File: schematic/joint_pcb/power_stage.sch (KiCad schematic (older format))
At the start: 36 parts, among them J2 Amp_Power, J3 Audio OUTPUT, Q1 IRF530A, Q2 IRF530A, Q3 IRF530A, Q4 IRF530A, U3 HIP4082IP

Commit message: Fixed PCB
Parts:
- Q1, Q2, Q3, Q4: symbol dk_Transistors-FETs-MOSFETs-Single:IRF540NPBF -> joint_pcb-rescue:IRF540NPBF-dk_Transistors-FETs-MOSFETs-Single
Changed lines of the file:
@@
 	3000 4350 3100 4350
 $Comp
-L dk_Transistors-FETs-MOSFETs-Single:IRF540NPBF Q2
+L joint_pcb-rescue:IRF540NPBF-dk_Transistors-FETs-MOSFETs-Single Q2
 U 1 1 61356BCC
 P 6500 4350
@@
 	4350 3950 5700 3950
 $Comp
-L dk_Transistors-FETs-MOSFETs-Single:IRF540NPBF Q3
+L joint_pcb-rescue:IRF540NPBF-dk_Transistors-FETs-MOSFETs-Single Q3
 U 1 1 61314458
 P 9650 2950
@@
 $EndComp
 $Comp
-L dk_Transistors-FETs-MOSFETs-Single:IRF540NPBF Q4
+L joint_pcb-rescue:IRF540NPBF-dk_Transistors-FETs-MOSFETs-Single Q4
 U 1 1 6132015F
 P 9650 4350
@@
 $EndComp
 $Comp
-L dk_Transistors-FETs-MOSFETs-Single:IRF540NPBF Q1
+L joint_pcb-rescue:IRF540NPBF-dk_Transistors-FETs-MOSFETs-Single Q1
 U 1 1 613134AB
 P 6500 2900

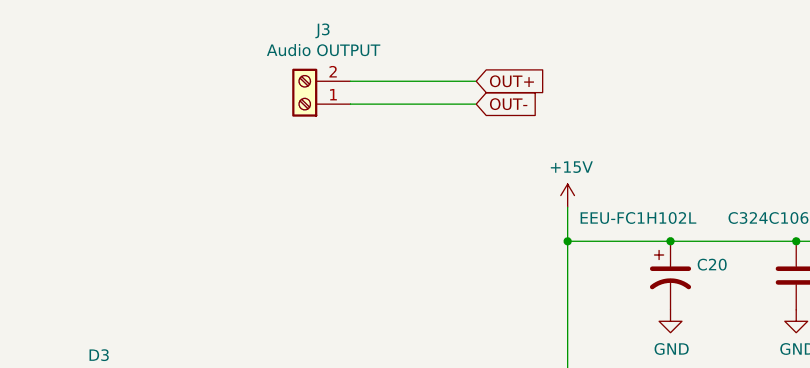
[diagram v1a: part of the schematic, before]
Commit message: finish layout for PCB
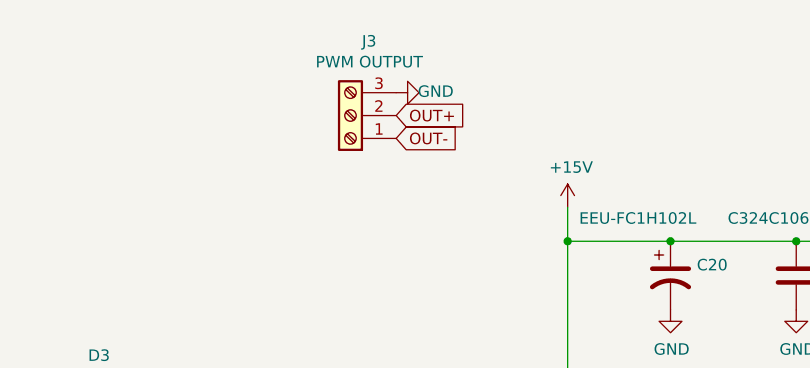
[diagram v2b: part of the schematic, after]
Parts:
- removed J3: Audio OUTPUT, TerminalBlock_Phoenix:TerminalBlock_Phoenix_PT-1,5-2-3.5-H_1x02_P3.50mm_Horizontal, symbol Connector:Screw_Terminal_01x02
- added J3: PWM OUTPUT, symbol Connector:Screw_Terminal_01x03
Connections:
- net GND: now also J3.3 (Pin_3)
- net OUT+: now also J3.2 (Pin_2)
- net OUT-: now also J3.1 (Pin_1)
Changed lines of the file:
@@
 $Descr A4 11693 8268
 encoding utf-8
-Sheet 3 4
+Sheet 3 3
 Title ""
 Date ""
@@
 Text GLabel 8750 3750 0    50   Output ~ 0
 OUT-
-Wire Wire Line
-	7050 1400 7600 1400
-Wire Wire Line
-	7050 1300 7600 1300
-$Comp
-L Connector:Screw_Terminal_01x02 J3
-U 1 1 613894BF
-P 6850 1400
-AR Path="/6133C499/613894BF" Ref="J3"  Part="1"
-AR Path="/6133C589/613894BF" Ref="J?"  Part="1"
-F 0 "J3" H 6768 1075 50  0000 C CNN
-F 1 "Audio OUTPUT" H 6768 1166 50  0000 C CNN
-F 2 "TerminalBlock_Phoenix:TerminalBlock_Phoenix_PT-1,5-2-3.5-H_1x02_P3.50mm_Horizontal" H 6850 1400 50  0001 C CNN
-F 3 "https://media.digikey.com/pdf/Data%20Sheets/Phoenix%20Contact%20PDFs/1935161.pdf" H 6850 1400 50  0001 C CNN
-F 4 "277-1667-ND" H 6850 1400 50  0001 C CNN "Digi-Key_PN"
-	1    6850 1400
-	-1   0    0    1
-$EndComp
-Text GLabel 7600 1400 2    50   Input ~ 0
+Text GLabel 7250 1550 2    50   Input ~ 0
 OUT-
-Text GLabel 7600 1300 2    50   Input ~ 0
+Text GLabel 7250 1450 2    50   Input ~ 0
 OUT+
+$Comp
+L Connector:Screw_Terminal_01x03 J3
+U 1 1 613ACDFA
+P 7050 1450
+F 0 "J3" H 6968 1125 50  0000 C CNN
+F 1 "PWM OUTPUT" H 6968 1216 50  0000 C CNN
+F 2 "" H 7050 1450 50  0001 C CNN
+F 3 "~" H 7050 1450 50  0001 C CNN
+	1    7050 1450
+	-1   0    0    1
+$EndComp
+$Comp
+L power:GND #PWR?
+U 1 1 613C0FA4
+P 7250 1350
+F 0 "#PWR?" H 7250 1100 50  0001 C CNN
+F 1 "GND" V 7255 1177 50  0000 C CNN
+F 2 "" H 7250 1350 50  0001 C CNN
+F 3 "" H 7250 1350 50  0001 C CNN
+	1    7250 1350
+	0    -1   -1   0
+$EndComp
 $EndSCHEMATC
